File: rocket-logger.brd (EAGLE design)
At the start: 58.5 x 62 mm, 61 parts, among them IC1 CC430F513X, U1 MAX1555, X1 0896BM15A0001, X2 USB-MICROB, X3 SMA-142-0701-801/806

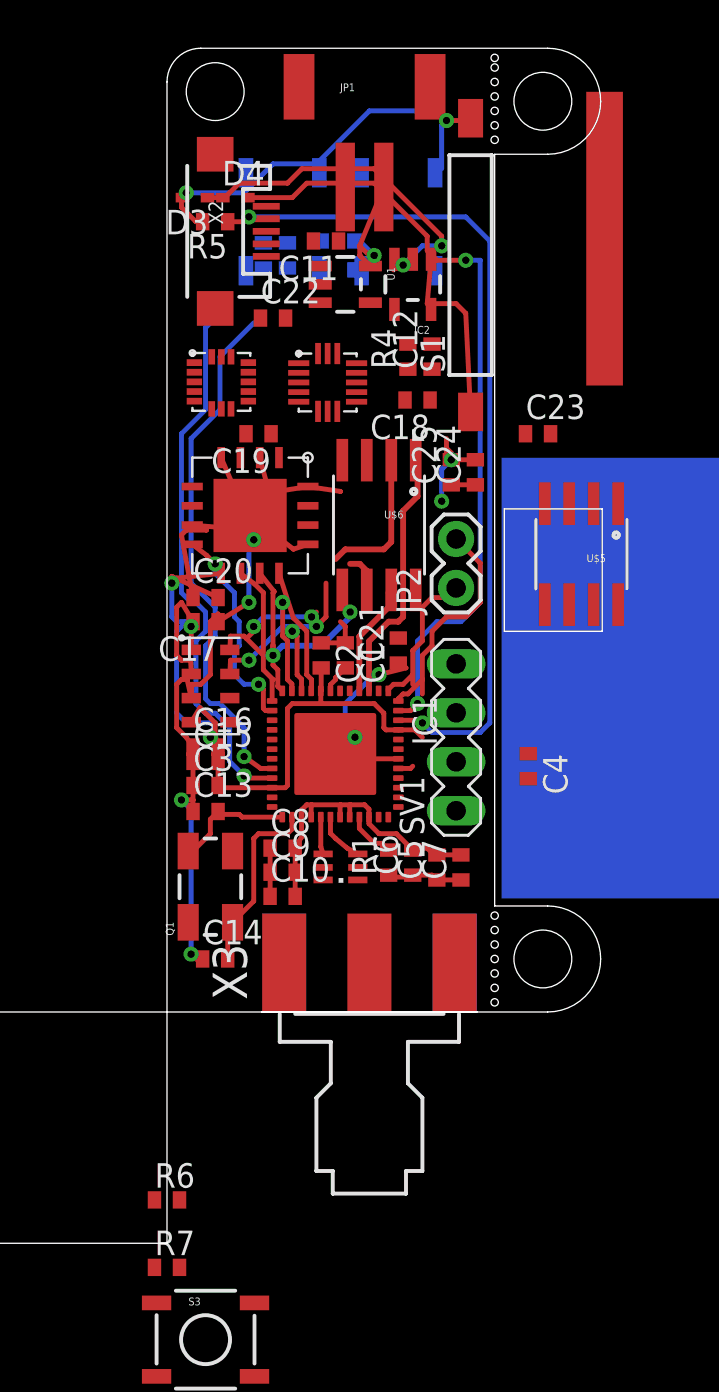
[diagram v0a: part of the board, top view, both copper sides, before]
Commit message: routing
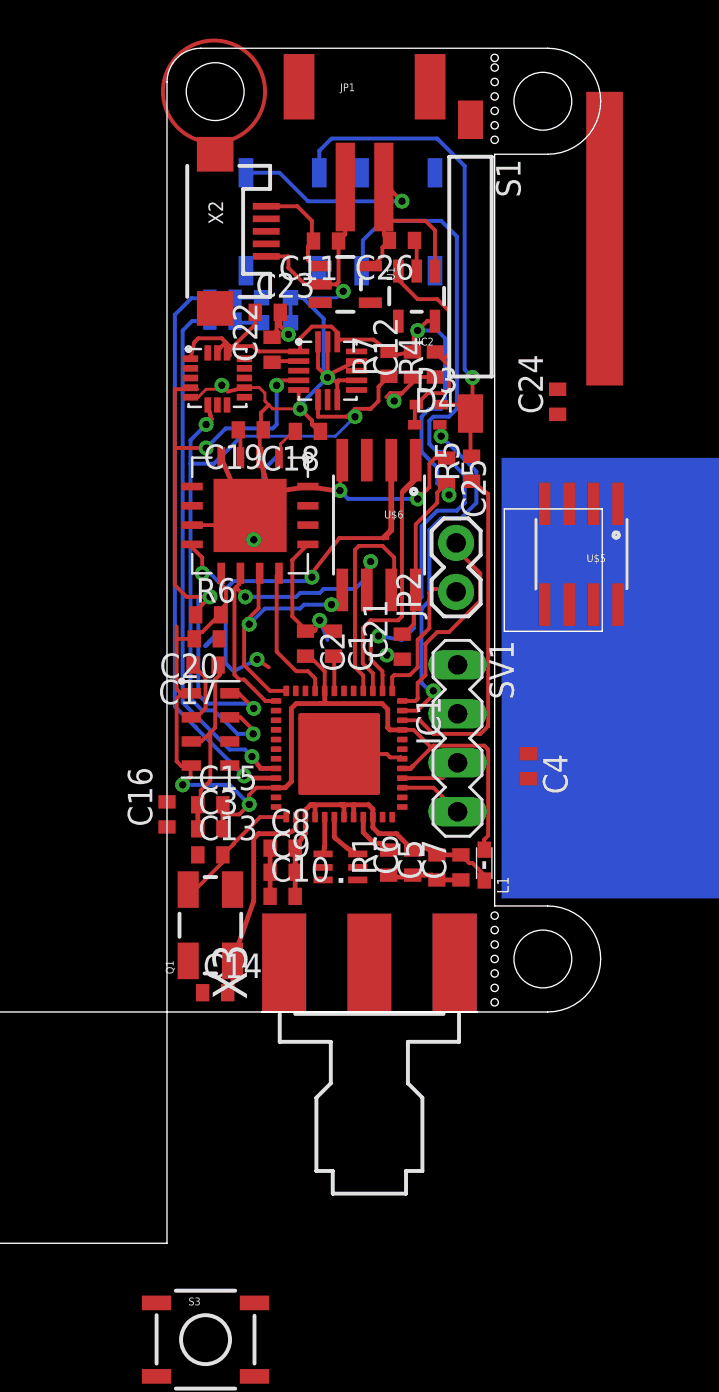
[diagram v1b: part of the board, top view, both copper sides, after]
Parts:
- added C26: (no value), resistor:C0402
- added L1: (no value), wuerth-elektronik:0603
- moved R7 48.3 mm to (11.5, 33.6), turned to 90 degrees
- moved R6 30.4 mm to (2.13, 20.6)
- moved R5 18.5 mm to (15.8, 28.2), turned to 90 degrees
- moved D3 16.1 mm to (13.5, 31.5), turned to 0 degrees
- moved D4 15.4 mm to (13.5, 30.5)
- moved C23 15.4 mm to (5.23, 36.3)
- moved C18 5.92 mm to (7.31, 30.1)
- moved C24 5.62 mm to (20.3, 31.7)
- moved LED2 5.38 mm to (5.66, 35.8), turned to 90 degrees
- moved R2 4.04 mm to (2.88, 37.0), turned to 180 degrees
- moved C16 4.03 mm to (0.00, 10.2), turned to 90 degrees
- moved R3 4.01 mm to (2.88, 35.8), turned to 180 degrees
- moved LED1 3.21 mm to (5.66, 37.1), turned to 90 degrees
- moved C13 2.26 mm to (2.25, 8.15)
- moved C15 2.26 mm to (2.25, 10.8)
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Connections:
- new net N$23: IC1.39, SV1.4
- new net N$26: IC1.40, SV1.3
- new net N$28: IC1.2, S4.3
- net +3V3: now also L1.2
- net AVCC_RF2: now also L1.1
- net GND: now also C26.1, LED1.C, LED2.C; no longer R2.2, R3.2
- net N$10: now also LED2.A, R3.2; no longer LED2.C, R3.1
- net N$16: now also R2.1; no longer LED1.A
- net N$17: now also R3.1; no longer LED2.A
- net N$2: now also C26.2
- net N$9: now also LED1.A, R2.2; no longer LED1.C, R2.1
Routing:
- net +3V3: track 48.3 -> 93.0 mm, vias 5 -> 4
- net N$28: track 0.00 -> 36.7 mm, vias 0 -> 1
- net GND: track 76.5 -> 110.7 mm, vias 6 -> 11
- net SWITCHON: track 44.4 -> 18.0 mm, vias 2 -> 0
- net SDA: track 11.9 -> 38.1 mm
- net SCL: track 12.7 -> 34.7 mm, vias 3 -> 4
- net KEEPON: track 40.7 -> 19.1 mm
- net CLK: track 9.41 -> 17.9 mm, vias 0 -> 2
- net N$25: track 18.4 -> 11.8 mm, vias 2 -> 0
- net HOLD: track 5.92 -> 11.7 mm
- net N$1: track 0.00 -> 5.63 mm
- net N$24: track 21.6 -> 26.5 mm, vias 2 -> 1
- net MISO: track 19.0 -> 23.9 mm, vias 2 -> 3
- net N$2: track 16.2 -> 19.6 mm
- net N$23: track 0.00 -> 3.38 mm
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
